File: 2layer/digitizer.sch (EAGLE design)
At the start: 40 parts, among them X1 SMA-142-0711-881/886, X2 SMA-142-0711-881/886

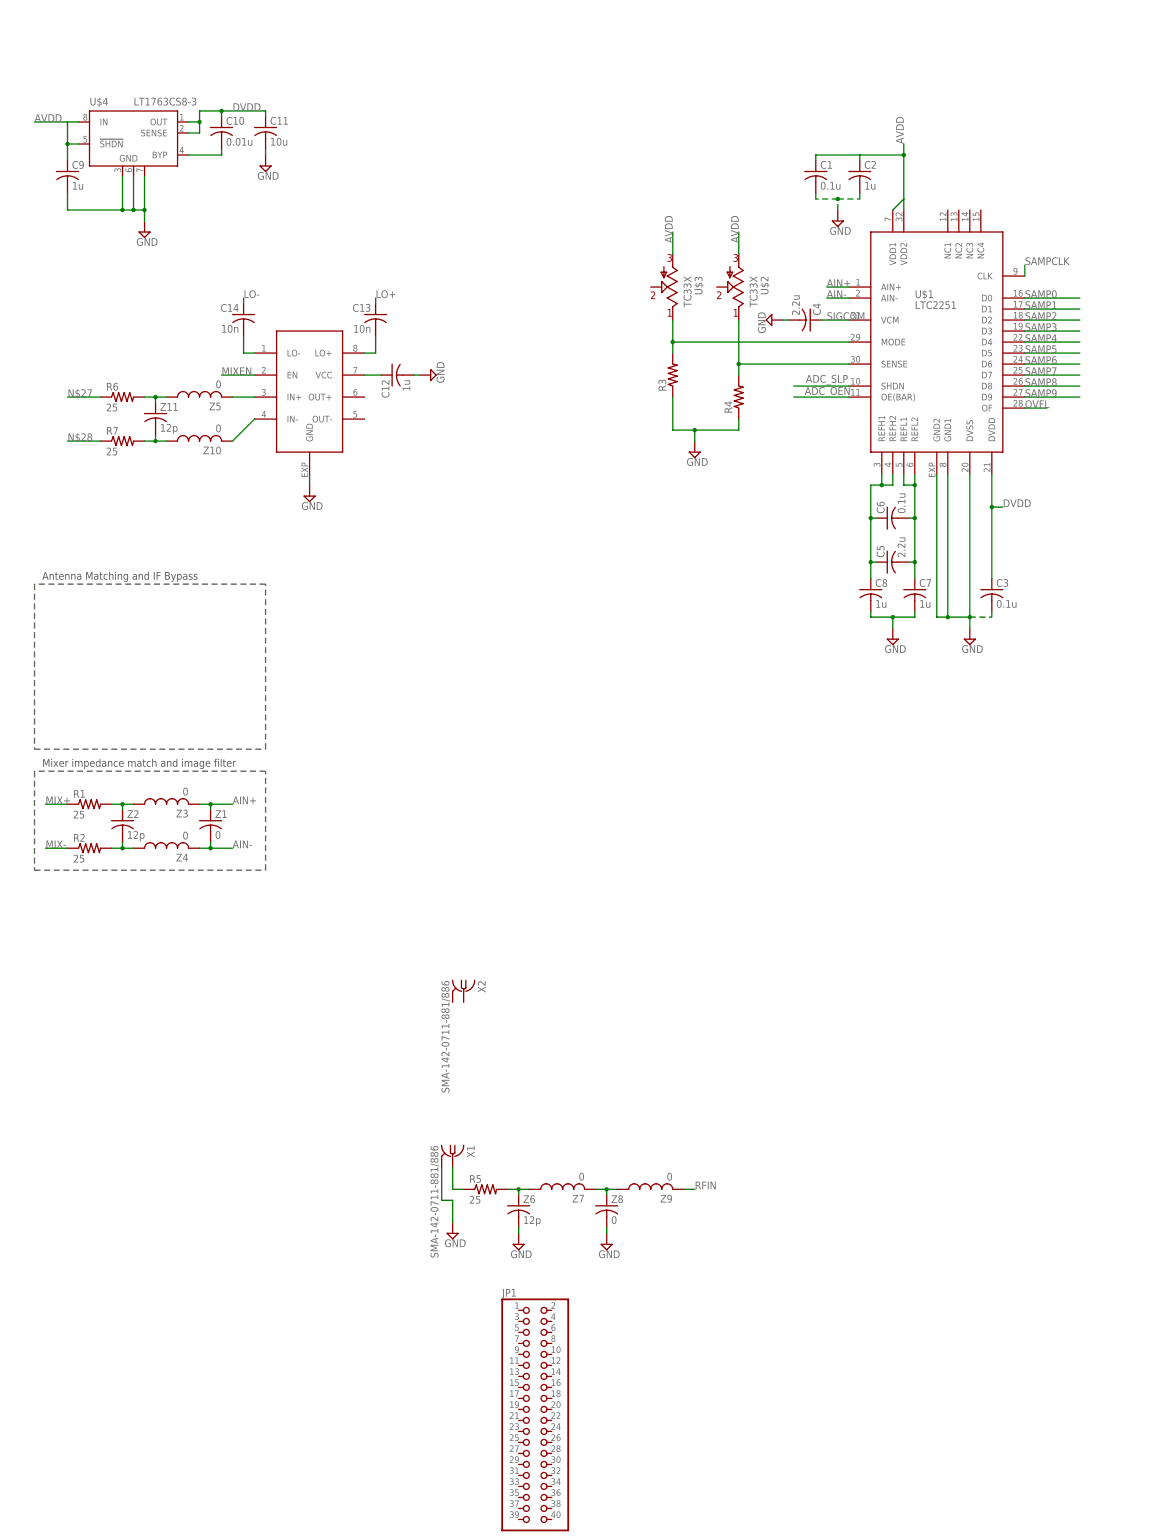
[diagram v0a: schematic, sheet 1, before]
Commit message: starting final layout
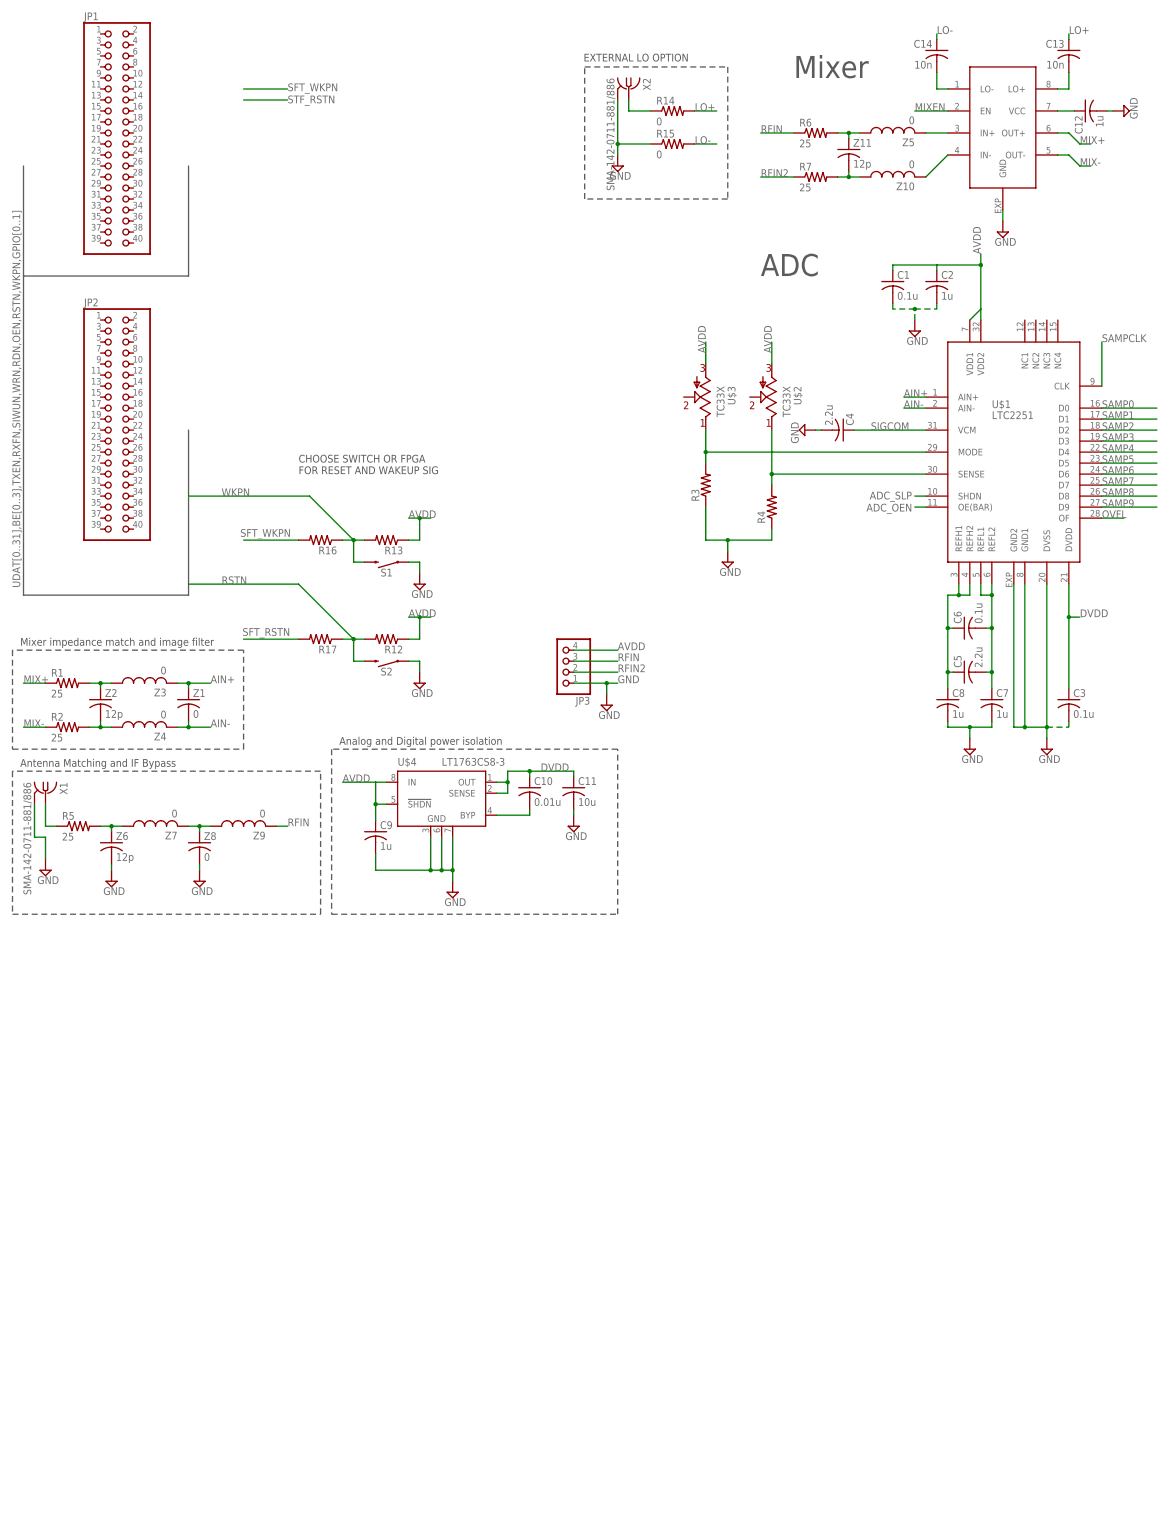
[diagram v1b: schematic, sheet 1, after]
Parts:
- added C15: (no value), rcl:C-USC0402
- added C16, C17: 18p, resistor:C-USC0402
- added C18, C19, C21: 0.1u, resistor:C-USC0402
- added C20: 1u, resistor:C-USC0402
- added C22: 4.7u, resistor:C-USC0402
- added IC1: FT601QQFN76, lt_ftdi_and_more:FT601QQFN76
- added JP2: (no value), pinhead:PINHD-2X20
- added JP3: (no value), pinhead:PINHD-1X4
- added R10, R12, R13, R16, R17: (no value), resistor:R-US_R0402
- added R11: (no value), resistor:R-US_V234/12
- added R14, R15: 0, resistor:R-US_R0805
- added S1, S2: MOMENTARY-SWITCH-SPST-SMD-6.0X3.5MM, SparkFun-Switches:MOMENTARY-SWITCH-SPST-SMD-6.0X3.5MM
- added U$6: USB3.0, components:USB3.0
- added U$7: CX3225SB_UKY1C-H1-16357-0045, components:CX3225SB_UKY1C-H1-16357-0045
- Z10, Z3, Z4, Z5: device components:L-US0805 -> components:L-US0402
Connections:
- removed net N$27: R6.1
- removed net N$28: R7.1
- new net BE0: IC1.BE_0
- new net BE1: IC1.BE_1
- new net BE2: IC1.BE_2
- new net BE3: IC1.BE_3
- new net D+: IC1.DP, U$6.D+
- new net D-: IC1.DM, U$6.D-
- new net FCLK: IC1.CLK
- new net GPIO0: IC1.GPIO0
- new net GPIO1: IC1.GPIO1
- new net N$11: C16.2, IC1.XI, U$7.1
- new net N$12: C17.2, IC1.XO, U$7.3
- new net N$13: IC1.RREF, R10.2, R11.2
- new net N$14: C18.2, U$6.SSTX+
- new net N$15: C19.2, U$6.SSTX-
- new net N$16: R14.1, X2.1
- new net OEN: IC1.OE_N
- new net OTG_ID: U$6.ID
- new net RDN: IC1.RD_N
- new net RFIN2: JP3.2, R7.1
- new net RSTN: IC1.RESET_N, R12.2, R17.1, S2.2
- new net RXFN: IC1.RXF_N
- new net SFT_RSTN: R17.2
- new net SFT_WKPN: R16.2
- new net SIWUN: IC1.SIWU_N
- new net SSRX+: IC1.RIDP, U$6.SSRX+
- new net SSRX-: IC1.RIDN, U$6.SSRX-
- new net SSTX+: C18.1, IC1.TODP
- new net SSTX-: C19.1, IC1.TODN
- new net TXEN: IC1.TXE_N
- new net UDAT0: IC1.DATA_0
- new net UDAT1: IC1.DATA_1
- new net UDAT10: IC1.DATA_10
- new net UDAT11: IC1.DATA_11
- new net UDAT12: IC1.DATA_12
- new net UDAT13: IC1.DATA_13
- new net UDAT14: IC1.DATA_14
- new net UDAT15: IC1.DATA_15
- new net UDAT16: IC1.DATA_16
- new net UDAT17: IC1.DATA_17
- new net UDAT18: IC1.DATA_18
- new net UDAT19: IC1.DATA_19
- new net UDAT2: IC1.DATA_2
- new net UDAT20: IC1.DATA_20
- new net UDAT21: IC1.DATA_21
- new net UDAT22: IC1.DATA_22
- new net UDAT23: IC1.DATA_23
- new net UDAT24: IC1.DATA_24
- new net UDAT25: IC1.DATA_25
- new net UDAT26: IC1.DATA_26
- new net UDAT27: IC1.DATA_27
- new net UDAT28: IC1.DATA_28
- new net UDAT29: IC1.DATA_29
- new net UDAT3: IC1.DATA_3
- new net UDAT30: IC1.DATA_30
- new net UDAT31: IC1.DATA_31
- new net UDAT4: IC1.DATA_4
- new net UDAT5: IC1.DATA_5
- new net UDAT6: IC1.DATA_6
- new net UDAT7: IC1.DATA_7
- new net UDAT8: IC1.DATA_8
- new net UDAT9: IC1.DATA_9
- new net V1REF: C15.2, C22.1, IC1.AVDD, IC1.DV10, IC1.VD10, IC1.VD10@1, IC1.VD10@2, IC1.VD10@3
- new net VBUS: IC1.VBUS, U$6.VBUS
- new net WKPN: IC1.WAKEUP_N, R13.2, R16.1, S1.2
- new net WRN: IC1.WR_N
- net AVDD: now also JP3.4, R12.1, R13.1
- net DVDD: now also C20.1, C21.1, IC1.VCC33, IC1.VCC33@1, IC1.VCC33@2, IC1.VCCIO, IC1.VCCIO@1, IC1.VCCIO@2, IC1.VCCIO@3, IC1.VDDA
- net GND: now also C15.1, C16.1, C17.1, C20.2, C21.2, C22.2, IC1.GND, IC1.GND@1, IC1.GND@2, IC1.GND@3, IC1.GND@4, JP3.1, R10.1, R11.1, R15.1, S1.1, S2.1, U$6.GND, U$6.GND-D, U$6.SHEILD1, U$6.SHEILD2, U$7.2, U$7.4, X2.2
- net LO+: now also R14.2
- net LO-: now also R15.2
- net MIX+: now also U$5.OUT+
- net MIX-: now also U$5.OUT-
- net RFIN: now also JP3.3, R6.1
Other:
- note added: "ADC"
- note added: "Analog and Digital power isolation"
- note added: "CHOOSE SWITCH OR FPGA FOR RESET AND WAKEUP SIG"
- note added: "EXTERNAL LO OPTION"
- note added: "Mixer"
- note added: "Stuff only one, dpt on pkg availability"
- moved on the sheet: C1, C10, C11, C12, C13, C14, C2, C3, C4, C5, C6, C7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
